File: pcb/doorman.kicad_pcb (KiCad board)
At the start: 4 copper layers, 37 x 37.2 mm, 62 parts, among them J1 USB-C Connector, J2 Screw Terminals, J3 3V3 Test Pad, J4 Extension Board Connector, J5 Siedle BUS RX Test Pad, J6 BUS Test Pad, J7 BUS RX Test Pad, J8 TX Test Pad, J9 RX Test Pad, Q1 BC847BPN, Q2 BC817-40, Q3 BC817-40, Q4 BC817-40, Q5 BC807-40, Q6 BC807-40, SW1 Button, SW2 Button, U2 AP63203WU, U3 GAQY252G3S, U4 ESP32-S3-MINI-1

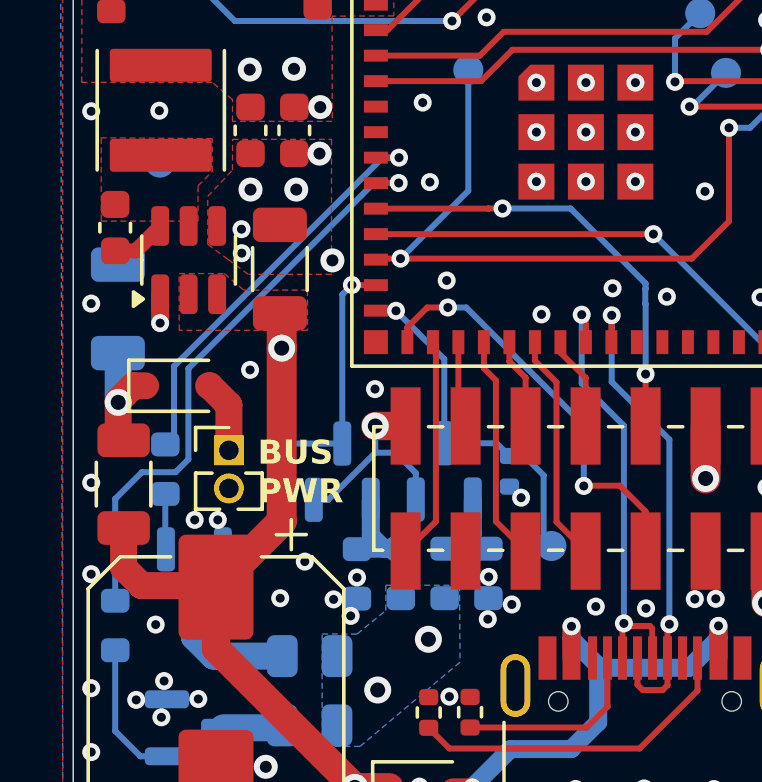
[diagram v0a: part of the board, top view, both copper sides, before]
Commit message: WIP
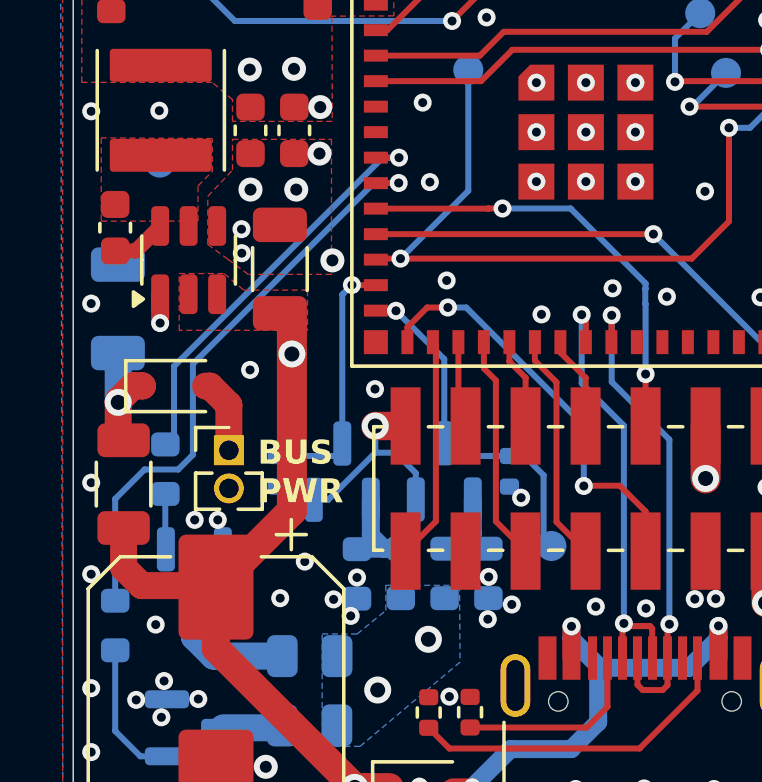
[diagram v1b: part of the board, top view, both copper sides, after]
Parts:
- moved D6 0.10 mm to (84.3, 57.5)
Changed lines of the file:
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@@
 	(footprint "Diode_SMD:D_SOD-323"
 		(layer "F.Cu")
-		(at 84.4125 57.47)
+		(at 84.3125 57.48)
 		(descr "SOD-323")
 		(tags "SOD-323")
@@
 	)
 	(segment
-		(start 86.14 58.11)
-		(end 86.14 59.62)
+		(start 85.3625 57.48)
+		(end 85.51 57.48)
 		(width 0.9)
 		(layer "F.Cu")
@@
 	)
 	(segment
-		(start 85.5 57.47)
-		(end 86.14 58.11)
+		(start 86.14 58.11)
+		(end 86.14 59.62)
 		(width 0.9)
 		(layer "F.Cu")
@@
 	)
 	(segment
-		(start 85.4625 57.47)
-		(end 85.5 57.47)
+		(start 85.51 57.48)
+		(end 86.14 58.11)
 		(width 0.9)
 		(layer "F.Cu")
@@
 	(segment
 		(start 82.45 58.0225)
-		(end 82.45 57.97)
+		(end 82.45 59.105)
 		(width 0.9)
 		(layer "F.Cu")
@@
 	)
 	(segment
-		(start 82.45 58.0225)
-		(end 82.45 59.105)
+		(start 82.95 57.47)
+		(end 83.2525 57.47)
 		(width 0.9)
 		(layer "F.Cu")
@@
 	)
 	(segment
-		(start 82.95 57.47)
-		(end 83.3625 57.47)
+		(start 83.2525 57.47)
+		(end 83.2625 57.48)
 		(width 0.9)
 		(layer "F.Cu")
@@
 		(net 26)
 	)
+	(segment
+		(start 82.45 58.0225)
+		(end 82.45 57.97)
+		(width 0.9)
+		(layer "F.Cu")
+		(net 26)
+	)
 	(via
 		(at 82.45 58.0225)
@@
 	)
 	(segment
-		(start 87.9 56.215)
-		(end 87.9 55.115001)
-		(width 1)
-		(layer "F.Cu")
-		(net 54)
-	)
-	(segment
 		(start 85.71 66.23)
 		(end 85.71 64.18)
@@
 	)
 	(segment
-		(start 85.36 64.13)
-		(end 83.23 64.13)
-		(width 0.9)
+		(start 85.71 64.17)
+		(end 85.71 64.18)
+		(width 1)
 		(layer "F.Cu")
 		(net 54)
 	)
 	(segment
-		(start 87.9 56.215)
-		(end 87.9 61.99)
-		(width 1)
+		(start 85.36 64.13)
+		(end 83.23 64.13)
+		(width 0.9)
 		(layer "F.Cu")
 		(net 54)
@@
 	)
 	(segment
-		(start 87.9 61.99)
-		(end 85.71 64.18)
-		(width 1)
-		(layer "F.Cu")
-		(net 54)
-	)
-	(segment
-		(start 87.9 55.115001)
-		(end 87.84 55.055001)
-		(width 1)
-		(layer "F.Cu")
-		(net 54)
-	)
-	(segment
 		(start 87.835 55.060001)
 		(end 87.835 55.130001)
@@
 	)
 	(segment
+		(start 88.24 55.455001)
+		(end 87.84 55.055001)
+		(width 1)
+		(layer "F.Cu")
+		(net 54)
+	)
+	(segment
 		(start 83.23 64.13)
 		(end 82.63 63.53)
@@
 	)
 	(segment
+		(start 88.24 56.41)
+		(end 88.24 55.455001)
+		(width 1)
+		(layer "F.Cu")
+		(net 54)
+	)
+	(segment
 		(start 90.335 70.855)
 		(end 91.4925 70.855)
@@
 		(net 54)
 	)
+	(segment
+		(start 88.24 56.41)
+		(end 88.24 61.64)
+		(width 1)
+		(layer "F.Cu")
+		(net 54)
+	)
+	(segment
+		(start 88.24 61.64)
+		(end 85.71 64.17)
+		(width 1)
+		(layer "F.Cu")
+		(net 54)
+	)
 	(via
 		(at 102.03 60.56)
@@
 	)
 	(via
-		(at 87.9 56.215)
+		(at 88.24 56.41)
 		(size 0.9)
 		(drill 0.5)
@@
 	)
 	(segment
-		(start 100.38 58.91)
-		(end 102.03 60.56)
+		(start 88.24 56.41)
+		(end 93.82 56.41)
 		(width 1)
 		(layer "In1.Cu")
@@
 	)
 	(segment
-		(start 93.625 56.215)
-		(end 96.32 58.91)
-		(width 1)
-		(layer "In1.Cu")
-		(net 54)
-	)
-	(segment
 		(start 111.895 70.87)
 		(end 111.91 70.855)
@@
 	)
 	(segment
-		(start 87.9 56.215)
-		(end 93.625 56.215)
+		(start 96.32 58.91)
+		(end 100.38 58.91)
 		(width 1)
 		(layer "In1.Cu")
@@
 	)
 	(segment
-		(start 96.32 58.91)
-		(end 100.38 58.91)
+		(start 93.82 56.41)
+		(end 96.32 58.91)
+		(width 1)
+		(layer "In1.Cu")
+		(net 54)
+	)
+	(segment
+		(start 100.38 58.91)
+		(end 102.03 60.56)
 		(width 1)
 		(layer "In1.Cu")
@@
 	(segment
 		(start 89.92 59.394999)
-		(end 88.165001 59.394999)
+		(end 89.92 59.81)
 		(width 0.2)
 		(layer "B.Cu")
@@
 	)
 	(segment
-		(start 88.165001 59.394999)
+		(start 89.92 59.81)
 		(end 87.75 59.81)
 		(width 0.2)
@@
 	)
 	(segment
+		(start 93.32 59.81)
+		(end 93.32 59.384999)
+		(width 0.2)
+		(layer "B.Cu")
+		(net 59)
+	)
+	(segment
 		(start 95.49 59.81)
 		(end 95.99 59.81)
@@
 	)
 	(segment
-		(start 95.064999 59.384999)
-		(end 93.32 59.384999)
+		(start 95.49 59.81)
+		(end 93.32 59.81)
 		(width 0.2)
 		(layer "B.Cu")
@@
 	)
 	(segment
-		(start 95.49 59.81)
-		(end 95.064999 59.384999)
-		(width 0.2)
-		(layer "B.Cu")
-		(net 59)
-	)
-	(segment
 		(start 96.63 62.55)
 		(end 96.89 62.81)
@@
 	)
 	(segment
-		(start 82.19 64.475)
-		(end 82.35 64.635)
+		(start 84.94 56.742958)
+		(end 84.94 59.77)
 		(width 0.2)
 		(layer "B.Cu")
@@
 	)
 	(segment
-		(start 91.8 50.71)
-		(end 90.972958 50.71)
+		(start 82.19 64.475)
+		(end 82.35 64.635)
 		(width 0.2)
 		(layer "B.Cu")
@@
 	)
 	(segment
-		(start 83.24 60.35)
-		(end 82.35 61.24)
+		(start 90.972958 50.71)
+		(end 84.94 56.742958)
 		(width 0.2)
 		(layer "B.Cu")
@@
 	)
 	(segment
-		(start 84.79 59.92)
-		(end 84.36 60.35)
+		(start 91.8 50.71)
+		(end 90.972958 50.71)
 		(width 0.2)
 		(layer "B.Cu")
@@
 	)
 	(segment
-		(start 84.79 56.892958)
-		(end 84.79 59.92)
+		(start 84.45 60.26)
+		(end 83.33 60.26)
 		(width 0.2)
 		(layer "B.Cu")
@@
 	)
 	(segment
-		(start 90.972958 50.71)
-		(end 84.79 56.892958)
+		(start 83.33 60.26)
+		(end 82.35 61.24)
 		(width 0.2)
 		(layer "B.Cu")
@@
 	)
 	(segment
-		(start 84.36 60.35)
-		(end 83.24 60.35)
+		(start 84.94 59.77)
+		(end 84.45 60.26)
 		(width 0.2)
 		(layer "B.Cu")
